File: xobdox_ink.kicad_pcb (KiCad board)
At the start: 2 copper layers, 22.9 x 34.8 mm, 34 parts, among them SW1 SW_Push, U1 XIAO-BLE, U2 EPD30

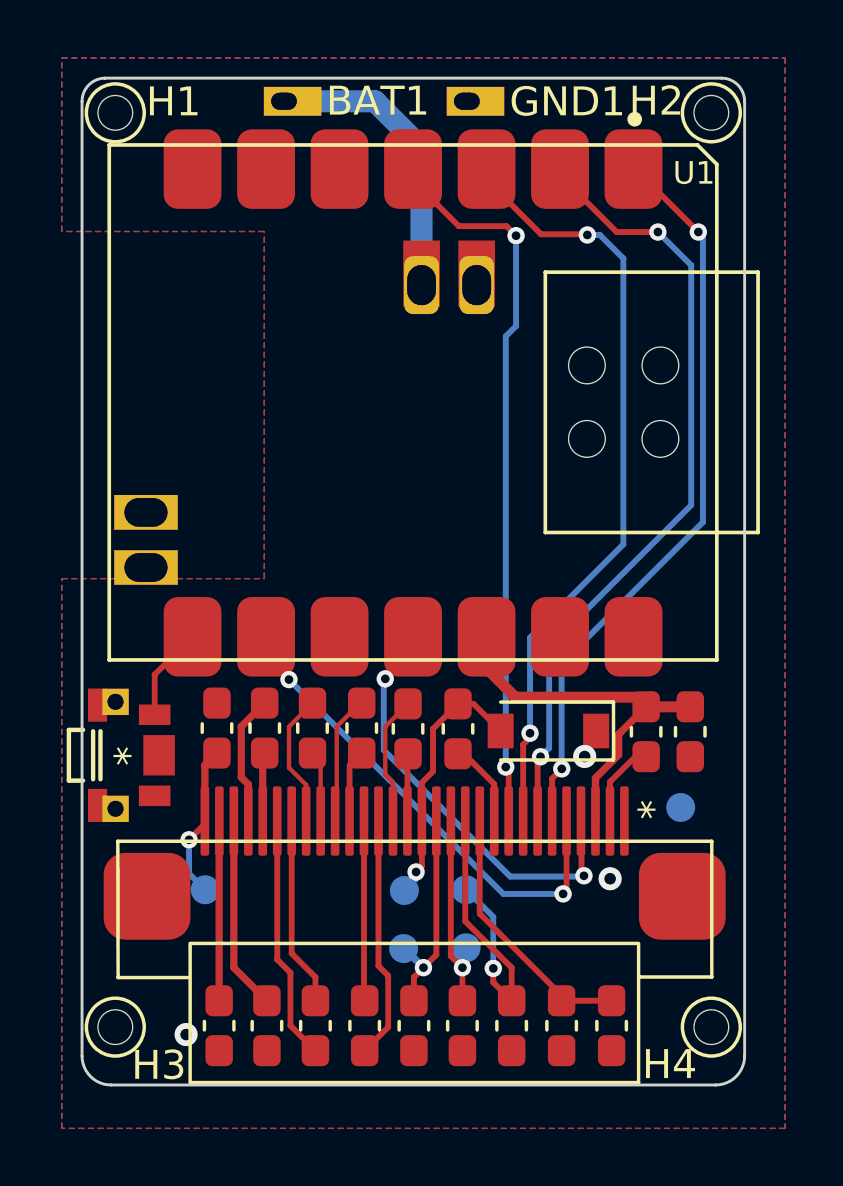
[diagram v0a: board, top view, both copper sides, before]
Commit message: add schematic and gerber
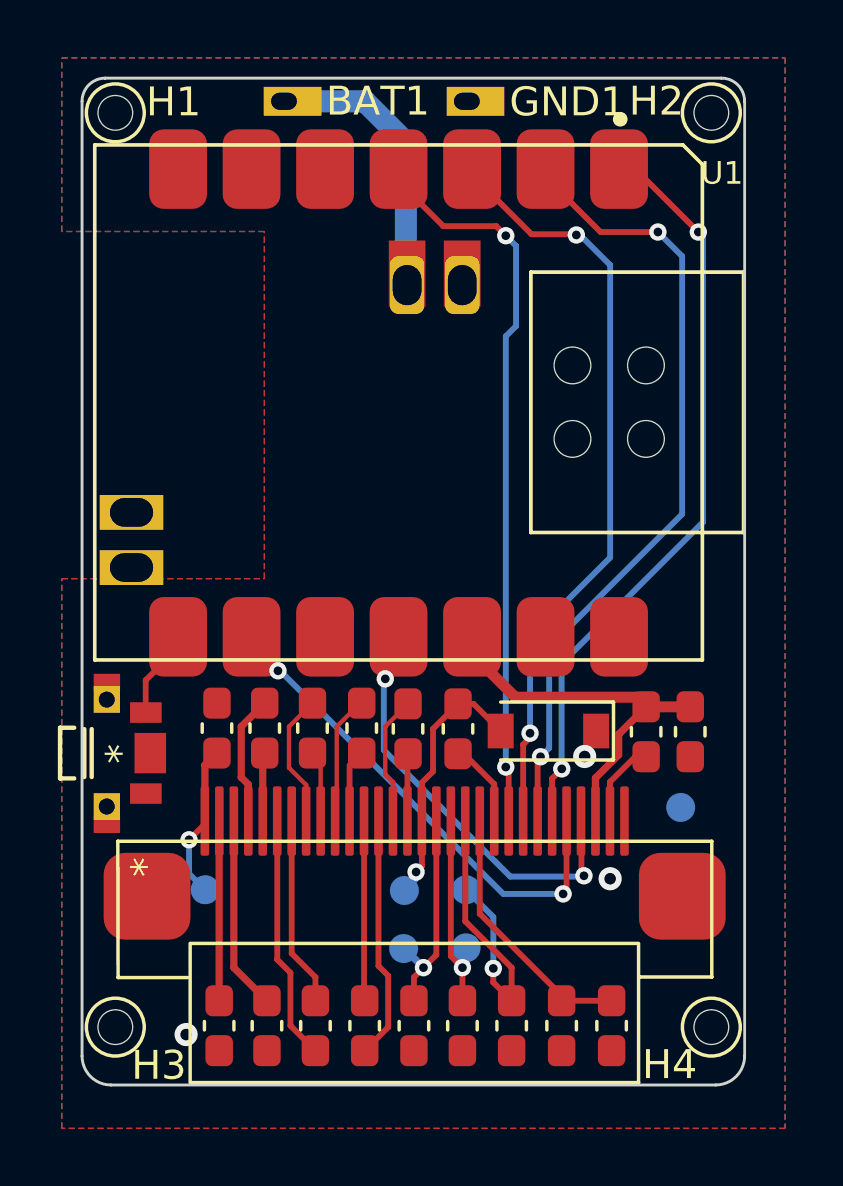
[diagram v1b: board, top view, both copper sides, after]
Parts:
- moved U1 0.50 mm to (170.3, 84.9)
- moved SW1 0.31 mm to (160.9, 97.0)
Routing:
- net /RES: track 27.1 -> 26.5 mm
